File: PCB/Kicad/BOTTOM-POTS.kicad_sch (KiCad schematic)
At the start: 17 parts

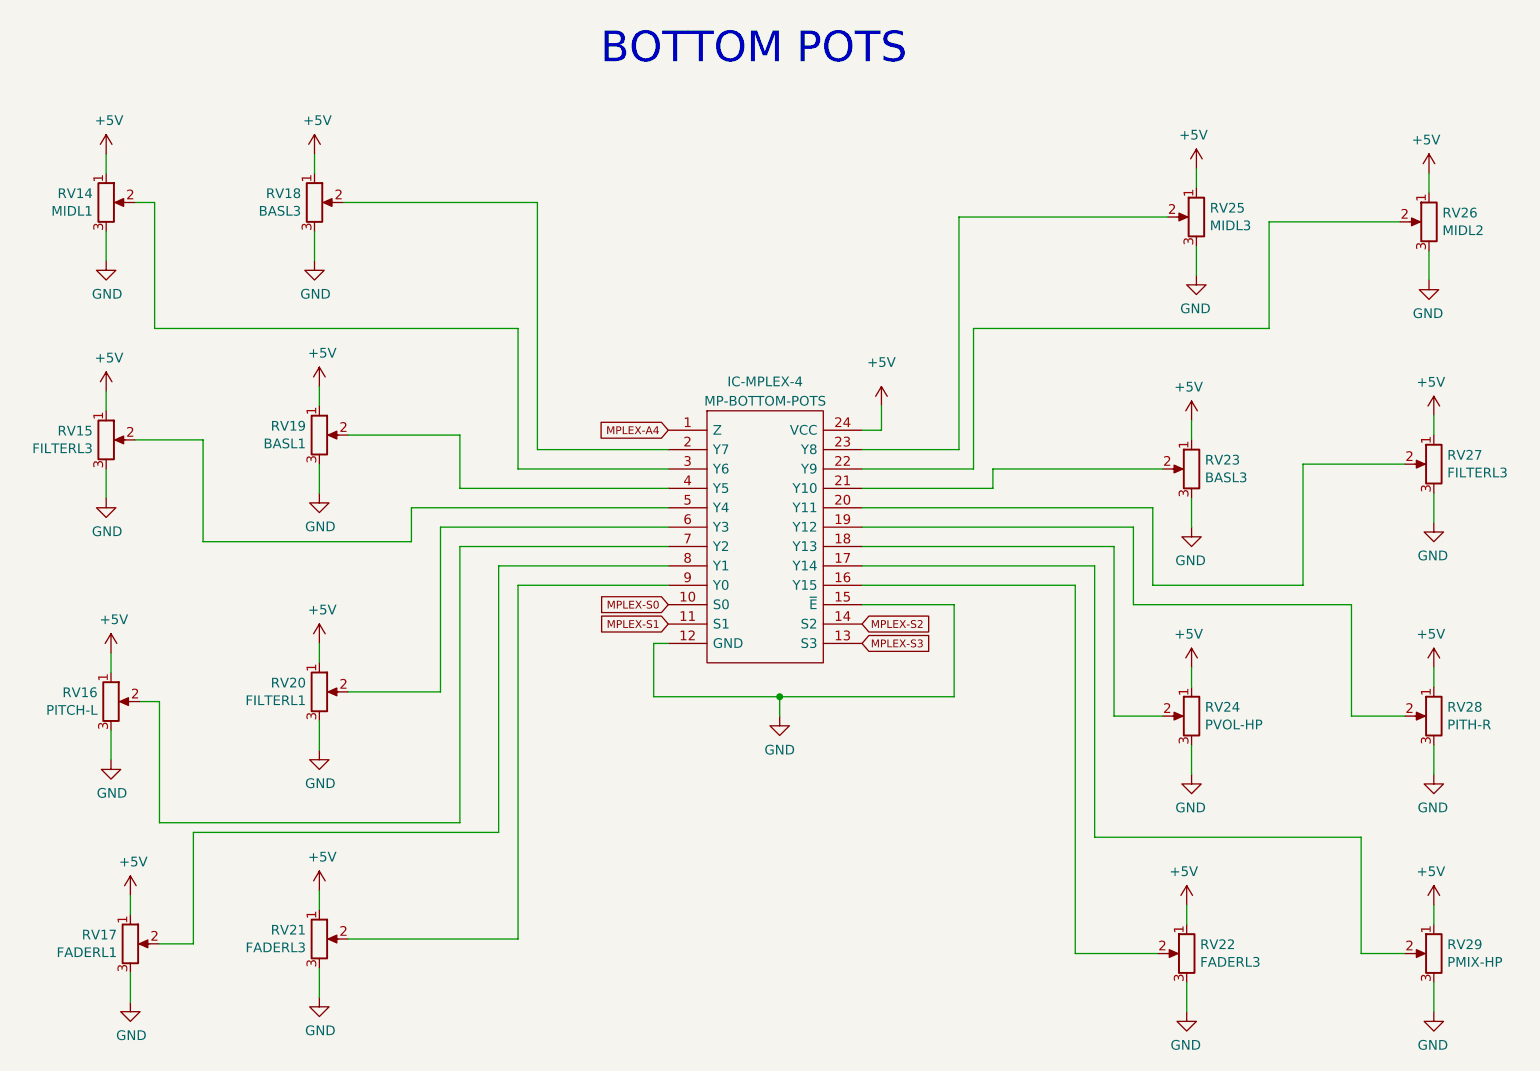
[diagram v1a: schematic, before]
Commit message: more routing
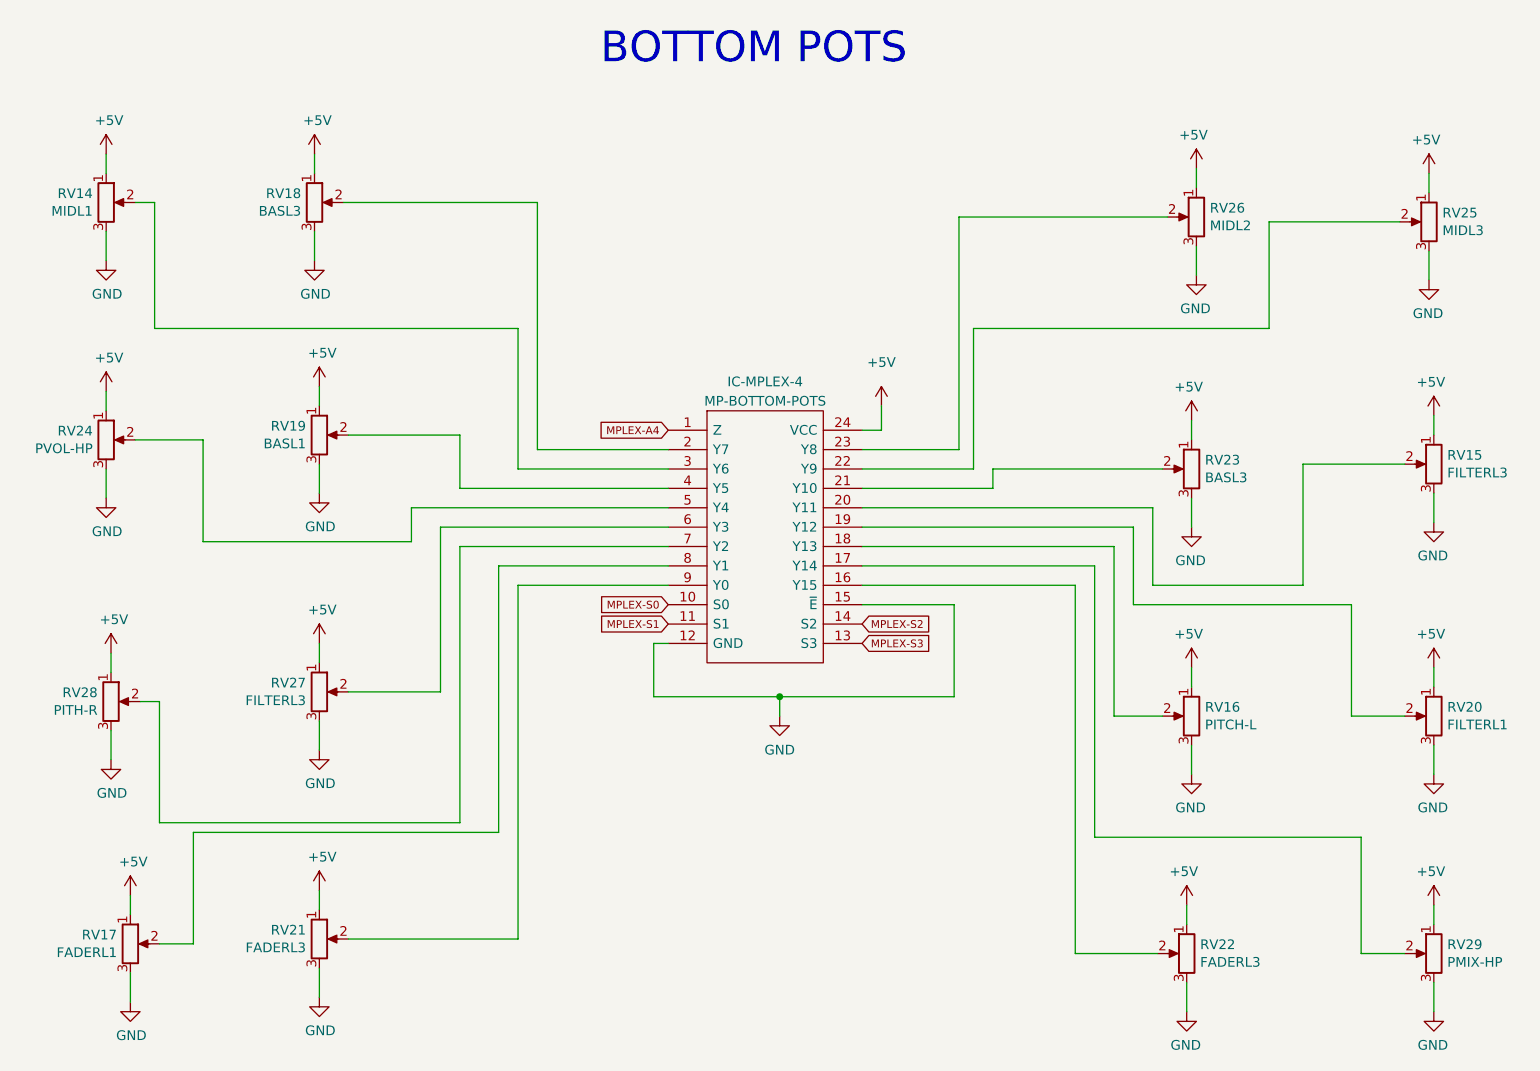
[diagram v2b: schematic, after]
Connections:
- net at IC-MPLEX-4.18 (Y13): now also RV16.2; no longer RV24.2
- net at IC-MPLEX-4.19 (Y12): now also RV20.2; no longer RV28.2
- net at IC-MPLEX-4.20 (Y11): now also RV15.2; no longer RV27.2
- net at IC-MPLEX-4.22 (Y9): now also RV25.2; no longer RV26.2
- net at IC-MPLEX-4.23 (Y8): now also RV26.2; no longer RV25.2
- net at IC-MPLEX-4.5 (Y4): now also RV24.2; no longer RV15.2
- net at IC-MPLEX-4.6 (Y3): now also RV27.2; no longer RV20.2
- net at IC-MPLEX-4.7 (Y2): now also RV28.2; no longer RV16.2
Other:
- moved on the sheet: RV15, RV16, RV20, RV24, RV25, RV26, RV27, RV28
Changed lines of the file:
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@@
-(kicad_sch (version 20210621) (generator eeschema)
+(kicad_sch (version 20210615) (generator eeschema)
   (paper "A4")
-  (junction (at 142.875 116.205) (diameter 0) (color 0 0 0 0))
+  (junction (at 142.875 116.205) (diameter 0.9144) (color 0 0 0 0))
   (wire (pts (xy 54.61 45.085) (xy 54.61 47.625))
     (stroke (width 0) (type solid) (color 0 0 0 0))
@@
   (symbol (lib_id "Device:R_Potentiometer") (at 54.61 82.55 0) (unit 1)
     (in_bom yes) (on_board yes)
-    (property "Reference" "RV15" (id 0) (at 52.8574 81.3816 0)
-      (effects (font (size 1.27 1.27)) (justify right))
-    )
-    (property "Value" "FILTERL3" (id 1) (at 52.8574 83.693 0)
+    (property "Reference" "RV24" (id 0) (at 52.8574 81.3816 0)
+      (effects (font (size 1.27 1.27)) (justify right))
+    )
+    (property "Value" "PVOL-HP" (id 1) (at 52.8574 83.693 0)
       (effects (font (size 1.27 1.27)) (justify right))
     )
@@
   (symbol (lib_id "Device:R_Potentiometer") (at 55.245 116.84 0) (unit 1)
     (in_bom yes) (on_board yes)
-    (property "Reference" "RV16" (id 0) (at 53.4924 115.6716 0)
-      (effects (font (size 1.27 1.27)) (justify right))
-    )
-    (property "Value" "PITCH-L" (id 1) (at 53.4924 117.983 0)
+    (property "Reference" "RV28" (id 0) (at 53.4924 115.6716 0)
+      (effects (font (size 1.27 1.27)) (justify right))
+    )
+    (property "Value" "PITH-R" (id 1) (at 53.4924 117.983 0)
       (effects (font (size 1.27 1.27)) (justify right))
     )
@@
   (symbol (lib_id "Device:R_Potentiometer") (at 82.55 115.57 0) (unit 1)
     (in_bom yes) (on_board yes)
-    (property "Reference" "RV20" (id 0) (at 80.7974 114.4016 0)
-      (effects (font (size 1.27 1.27)) (justify right))
-    )
-    (property "Value" "FILTERL1" (id 1) (at 80.7974 116.713 0)
+    (property "Reference" "RV27" (id 0) (at 80.7974 114.4016 0)
+      (effects (font (size 1.27 1.27)) (justify right))
+    )
+    (property "Value" "FILTERL3" (id 1) (at 80.7974 116.713 0)
       (effects (font (size 1.27 1.27)) (justify right))
     )
@@
   (symbol (lib_id "Device:R_Potentiometer") (at 196.85 118.745 0) (mirror y) (unit 1)
     (in_bom yes) (on_board yes)
-    (property "Reference" "RV24" (id 0) (at 198.6026 117.5766 0)
-      (effects (font (size 1.27 1.27)) (justify right))
-    )
-    (property "Value" "PVOL-HP" (id 1) (at 198.6026 119.888 0)
-      (effects (font (size 1.27 1.27)) (justify right))
-    )
-    (property "Footprint" "Library:Potentiometer_Bourns_PTV09A-1_Single_Vertical" (id 2) (at 196.85 118.745 0)
+    (property "Reference" "RV16" (id 0) (at 198.6026 117.5766 0)
+      (effects (font (size 1.27 1.27)) (justify right))
+    )
+    (property "Value" "PITCH-L" (id 1) (at 198.6026 119.888 0)
+      (effects (font (size 1.27 1.27)) (justify right))
+    )
+    (property "Footprint" "Library:fader-L75" (id 2) (at 196.85 118.745 0)
       (effects (font (size 1.27 1.27)) hide)
     )
@@
   (symbol (lib_id "Device:R_Potentiometer") (at 197.485 53.34 0) (mirror y) (unit 1)
     (in_bom yes) (on_board yes)
-    (property "Reference" "RV25" (id 0) (at 199.2376 52.1716 0)
-      (effects (font (size 1.27 1.27)) (justify right))
-    )
-    (property "Value" "MIDL3" (id 1) (at 199.2376 54.483 0)
+    (property "Reference" "RV26" (id 0) (at 199.2376 52.1716 0)
+      (effects (font (size 1.27 1.27)) (justify right))
+    )
+    (property "Value" "MIDL2" (id 1) (at 199.2376 54.483 0)
       (effects (font (size 1.27 1.27)) (justify right))
     )
@@
   (symbol (lib_id "Device:R_Potentiometer") (at 227.965 53.975 0) (mirror y) (unit 1)
     (in_bom yes) (on_board yes)
-    (property "Reference" "RV26" (id 0) (at 229.7176 52.8066 0)
-      (effects (font (size 1.27 1.27)) (justify right))
-    )
-    (property "Value" "MIDL2" (id 1) (at 229.7176 55.118 0)
+    (property "Reference" "RV25" (id 0) (at 229.7176 52.8066 0)
+      (effects (font (size 1.27 1.27)) (justify right))
+    )
+    (property "Value" "MIDL3" (id 1) (at 229.7176 55.118 0)
       (effects (font (size 1.27 1.27)) (justify right))
     )
@@
   (symbol (lib_id "Device:R_Potentiometer") (at 228.6 85.725 0) (mirror y) (unit 1)
     (in_bom yes) (on_board yes)
-    (property "Reference" "RV27" (id 0) (at 230.3526 84.5566 0)
+    (property "Reference" "RV15" (id 0) (at 230.3526 84.5566 0)
       (effects (font (size 1.27 1.27)) (justify right))
     )
@@
   (symbol (lib_id "Device:R_Potentiometer") (at 228.6 118.745 0) (mirror y) (unit 1)
     (in_bom yes) (on_board yes)
-    (property "Reference" "RV28" (id 0) (at 230.3526 117.5766 0)
-      (effects (font (size 1.27 1.27)) (justify right))
-    )
-    (property "Value" "PITH-R" (id 1) (at 230.3526 119.888 0)
-      (effects (font (size 1.27 1.27)) (justify right))
-    )
-    (property "Footprint" "Library:fader-L75" (id 2) (at 228.6 118.745 0)
-      (effects (font (size 1.27 1.27)) hide)
-    )
+    (property "Reference" "RV20" (id 0) (at 230.3526 117.5766 0)
+      (effects (font (size 1.27 1.27)) (justify right))
+    )
+    (property "Value" "FILTERL1" (id 1) (at 230.3526 119.888 0)
+      (effects (font (size 1.27 1.27)) (justify right))
+    )
+    (property "Footprint" "Library:Potentiometer_Bourns_PTV09A-1_Single_Vertical" (id 2) (at 228.6 118.745 0)
+      (effects (font (size 1.27 1.27)) hide)
+    )

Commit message: update schematic
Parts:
- IC-MPLEX-4: footprint Library:SOIC-24W_7.5x15.4mm_P1.27mm -> Package_SO:SOIC-24W_7.5x15.4mm_P1.27mm
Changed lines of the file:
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@@
     (property "Reference" "IC-MPLEX-4" (id 0) (at 140.97 74.93 0))
     (property "Value" "MP-BOTTOM-POTS" (id 1) (at 140.97 77.47 0))
-    (property "Footprint" "Library:SOIC-24W_7.5x15.4mm_P1.27mm" (id 2) (at 149.86 78.74 0)
+    (property "Footprint" "Package_SO:SOIC-24W_7.5x15.4mm_P1.27mm" (id 2) (at 149.86 78.74 0)
       (effects (font (size 1.27 1.27)) (justify left) hide)
     )
